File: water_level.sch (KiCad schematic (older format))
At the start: 14 parts, among them U1 LTV-847

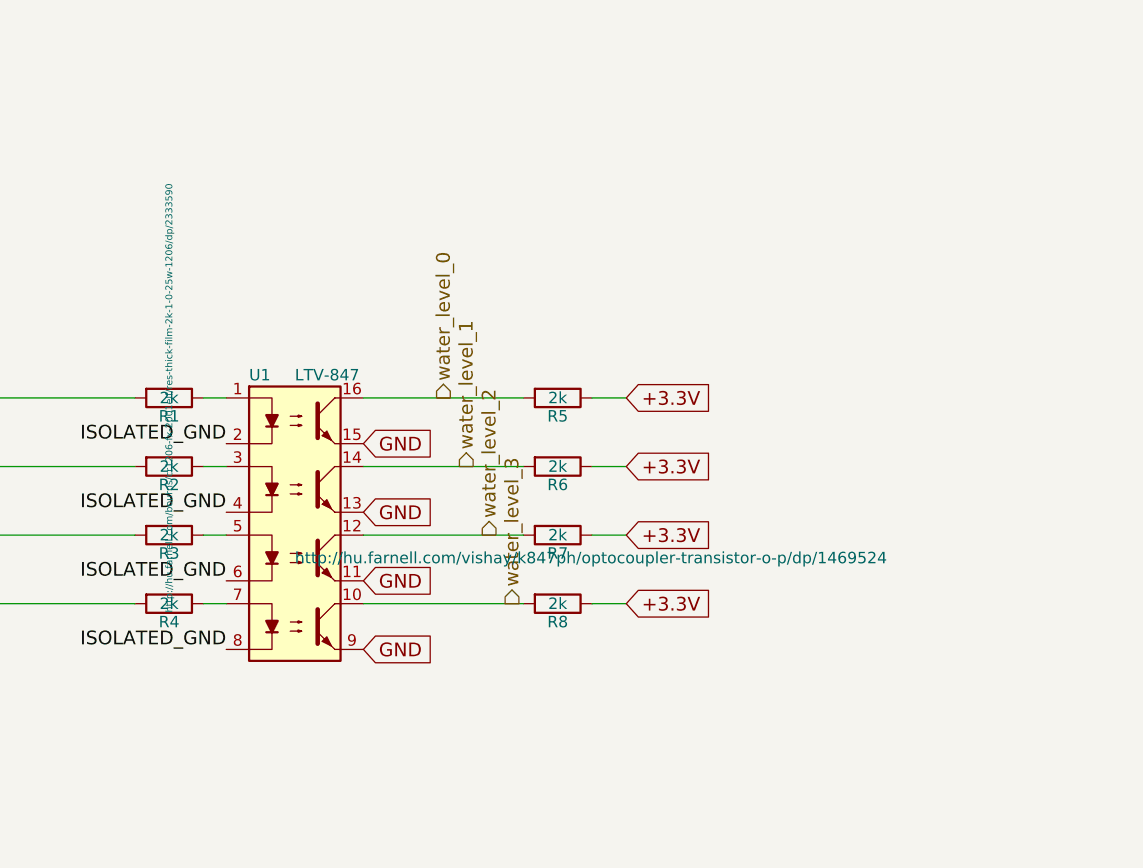
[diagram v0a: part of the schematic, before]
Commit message: stash commit before the revision of the parts
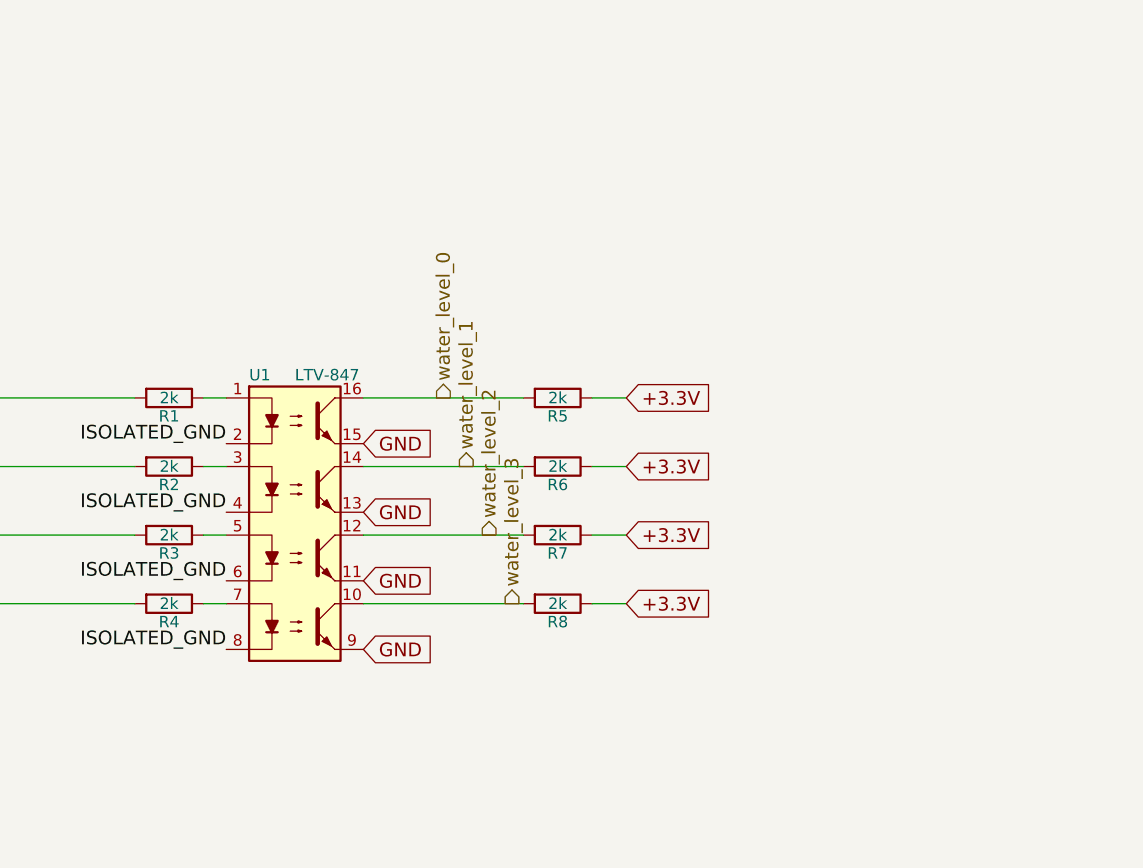
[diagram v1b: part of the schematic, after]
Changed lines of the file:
@@
 F 1 "LTV-847" H 7350 3850 50  0000 L CNN
 F 2 "Housings_SOIC:SOIC-16_3.9x9.9mm_Pitch1.27mm" H 7150 2550 50  0001 L CIN
-F 3 "http://hu.farnell.com/vishay/k847ph/optocoupler-transistor-o-p/dp/1469524" H 7350 3050 50  0000 L CNN
+F 3 "http://hu.farnell.com/vishay/k847ph/optocoupler-transistor-o-p/dp/1469524" H 7350 3050 50  0001 L CNN
 	1    7350 3150
 	1    0    0    -1
@@
 F 1 "2k" V 6800 2550 50  0000 C CNN
 F 2 "Resistors_SMD:R_1206_HandSoldering" V 6730 2550 30  0001 C CNN
-F 3 "http://hu.farnell.com/bourns/cr1206-fx-2001elf/res-thick-film-2k-1-0-25w-1206/dp/2333590" H 6800 2550 30  0000 C CNN
+F 3 "http://hu.farnell.com/bourns/cr1206-fx-2001elf/res-thick-film-2k-1-0-25w-1206/dp/2333590" H 6800 2550 30  0001 C CNN
 	1    6800 2550
 	0    1    1    0
@@
 +5V
 $Comp
+L Water_Level_Sensor_Connector SENS_1
+U 1 1 592601C6
+P 3600 2600
+F 0 "SENS_1" H 3450 1500 60  0000 C CNN
+F 1 "Water_Level_Sensor_Connector" H 3600 2600 60  0000 C CNN
+F 2 "Connectors_Terminal_Blocks:TerminalBlock_WAGO-804_RM5mm_5pol" H 3600 2600 60  0001 C CNN
+F 3 "http://hu.farnell.com/wago/2604-1105/tb-wire-to-brd-5pos-12awg/dp/2749668" H 3600 2600 60  0001 C CNN
+	1    3600 2600
+	1    0    0    -1
+$EndComp
+$Comp
+L Water_Level_Sensor_Connector SENS_3
+U 1 1 59260240
+P 3600 5150
+F 0 "SENS_3" H 3450 4050 60  0000 C CNN
+F 1 "Water_Level_Sensor_Connector" H 3600 5150 60  0000 C CNN
+F 2 "Connectors_Terminal_Blocks:TerminalBlock_WAGO-804_RM5mm_5pol" H 3600 5150 60  0001 C CNN
+F 3 "http://hu.farnell.com/wago/2604-1105/tb-wire-to-brd-5pos-12awg/dp/2749668" H 3600 5150 60  0001 C CNN
+	1    3600 5150
+	1    0    0    -1
+$EndComp
+$Comp
+L Water_Level_Sensor_Connector SENS_4
+U 1 1 592602C7
+P 3600 6400
+F 0 "SENS_4" H 3450 5300 60  0000 C CNN
+F 1 "Water_Level_Sensor_Connector" H 3600 6400 60  0000 C CNN
+F 2 "Connectors_Terminal_Blocks:TerminalBlock_WAGO-804_RM5mm_5pol" H 3600 6400 60  0001 C CNN
+F 3 "http://hu.farnell.com/wago/2604-1105/tb-wire-to-brd-5pos-12awg/dp/2749668" H 3600 6400 60  0001 C CNN
+	1    3600 6400
+	1    0    0    -1
+$EndComp
+Wire Wire Line
+	7650 2550 8350 2550
+Wire Wire Line
+	7650 2850 8350 2850
+Wire Wire Line
+	7650 3150 8350 3150
+Wire Wire Line
+	7650 3450 8350 3450
+Wire Wire Line
+	8800 2550 8650 2550
+Wire Wire Line
+	8800 2850 8650 2850
+Wire Wire Line
+	8800 3150 8650 3150
+Wire Wire Line
+	8800 3450 8650 3450
+Wire Wire Line
+	6950 3450 7050 3450
+Wire Wire Line
+	6950 3150 7050 3150
+Wire Wire Line
+	6950 2850 7050 2850
+Wire Wire Line
+	6950 2550 7050 2550
+Text GLabel 7650 3650 2    60   Input ~ 0
+GND
+Text GLabel 7650 3350 2    60   Input ~ 0
+GND
+Text GLabel 7650 3050 2    60   Input ~ 0
+GND
+Text GLabel 7650 2750 2    60   Input ~ 0
+GND
+Text GLabel 8800 2550 2    60   Input ~ 0
++3.3V
+Text GLabel 8800 2850 2    60   Input ~ 0
++3.3V
+Text GLabel 8800 3150 2    60   Input ~ 0
++3.3V
+Text GLabel 8800 3450 2    60   Input ~ 0
++3.3V
+Text Label 2000 1200 0    60   ~ 0
+ISOLATED_GND
+Text Label 3100 2850 2    60   ~ 0
+ISOLATED_GND
+Text Label 3100 4100 2    60   ~ 0
+ISOLATED_GND
+Text Label 3100 5400 2    60   ~ 0
+ISOLATED_GND
+Text Label 3100 6650 2    60   ~ 0
+ISOLATED_GND
+Text Label 7050 2750 2    60   ~ 0
+ISOLATED_GND
+Text Label 7050 3050 2    60   ~ 0
+ISOLATED_GND
+Text Label 7050 3350 2    60   ~ 0
+ISOLATED_GND
+Text Label 7050 3650 2    60   ~ 0
+ISOLATED_GND
+Text Label 2000 1450 0    60   ~ 0
+ISOLATED_+12V
+Text Label 3100 3000 2    60   ~ 0
+ISOLATED_+12V
+Text Label 3100 4250 2    60   ~ 0
+ISOLATED_+12V
+Text Label 3100 5550 2    60   ~ 0
+ISOLATED_+12V
+Text Label 3100 6800 2    60   ~ 0
+ISOLATED_+12V
+Text Label 3100 3150 2    60   ~ 0
+ISOLATED_+12V
+Text Label 3100 4400 2    60   ~ 0
+ISOLATED_+12V
+Text Label 3100 5700 2    60   ~ 0
+ISOLATED_+12V
+Text Label 3100 6950 2    60   ~ 0
+ISOLATED_+12V
+Wire Wire Line
+	3800 3300 4650 3300
+Wire Wire Line
+	4650 3300 4650 2550
+Wire Wire Line
+	4650 2550 6650 2550
+Wire Wire Line
+	3800 4550 4850 4550
+Wire Wire Line
+	4850 4550 4850 2850
+Wire Wire Line
+	4850 2850 6650 2850
+Wire Wire Line
+	3800 5850 5050 5850
+Wire Wire Line
+	5050 5850 5050 3150
+Wire Wire Line
+	5050 3150 6650 3150
+Wire Wire Line
+	3800 7100 5250 7100
+Wire Wire Line
+	5250 7100 5250 3450
+Wire Wire Line
+	5250 3450 6650 3450
+$Comp
 L Water_Level_Sensor_Connector SENS_2
 U 1 1 5925F963
@@
 F 1 "Water_Level_Sensor_Connector" H 3600 3850 60  0000 C CNN
 F 2 "Connectors_Terminal_Blocks:TerminalBlock_WAGO-804_RM5mm_5pol" H 3600 3850 60  0001 C CNN
-F 3 "http://hu.farnell.com/wago/2092-1375/terminal-block-wire-to-brd-5pos/dp/2352416" H 3600 3850 60  0001 C CNN
+F 3 "http://hu.farnell.com/wago/2604-1105/tb-wire-to-brd-5pos-12awg/dp/2749668" H 3600 3850 60  0001 C CNN
 	1    3600 3850
 	1    0    0    -1
 $EndComp
-$Comp
-L Water_Level_Sensor_Connector SENS_1
-U 1 1 592601C6
-P 3600 2600
-F 0 "SENS_1" H 3450 1500 60  0000 C CNN
-F 1 "Water_Level_Sensor_Connector" H 3600 2600 60  0000 C CNN
-F 2 "Connectors_Terminal_Blocks:TerminalBlock_WAGO-804_RM5mm_5pol" H 3600 2600 60  0001 C CNN
-F 3 "http://hu.farnell.com/wago/2092-1375/terminal-block-wire-to-brd-5pos/dp/2352416" H 3600 2600 60  0001 C CNN
-	1    3600 2600
-	1    0    0    -1
-$EndComp
-$Comp
-L Water_Level_Sensor_Connector SENS_3
-U 1 1 59260240
-P 3600 5150
-F 0 "SENS_3" H 3450 4050 60  0000 C CNN
-F 1 "Water_Level_Sensor_Connector" H 3600 5150 60  0000 C CNN
-F 2 "Connectors_Terminal_Blocks:TerminalBlock_WAGO-804_RM5mm_5pol" H 3600 5150 60  0001 C CNN
-F 3 "http://hu.farnell.com/wago/2092-1375/terminal-block-wire-to-brd-5pos/dp/2352416" H 3600 5150 60  0001 C CNN
-	1    3600 5150
-	1    0    0    -1
-$EndComp
-$Comp
-L Water_Level_Sensor_Connector SENS_4
-U 1 1 592602C7
-P 3600 6400
-F 0 "SENS_4" H 3450 5300 60  0000 C CNN
-F 1 "Water_Level_Sensor_Connector" H 3600 6400 60  0000 C CNN
-F 2 "Connectors_Terminal_Blocks:TerminalBlock_WAGO-804_RM5mm_5pol" H 3600 6400 60  0001 C CNN
-F 3 "http://hu.farnell.com/wago/2092-1375/terminal-block-wire-to-brd-5pos/dp/2352416" H 3600 6400 60  0001 C CNN
-	1    3600 6400
-	1    0    0    -1
-$EndComp
-Wire Wire Line
-	7650 2550 8350 2550
-Wire Wire Line
-	7650 2850 8350 2850
-Wire Wire Line
-	7650 3150 8350 3150
-Wire Wire Line
-	7650 3450 8350 3450
-Wire Wire Line
-	8800 2550 8650 2550
-Wire Wire Line
-	8800 2850 8650 2850
-Wire Wire Line
-	8800 3150 8650 3150
-Wire Wire Line
-	8800 3450 8650 3450
-Wire Wire Line
-	6950 3450 7050 3450
-Wire Wire Line
-	6950 3150 7050 3150
-Wire Wire Line
-	6950 2850 7050 2850
-Wire Wire Line
-	6950 2550 7050 2550
-Text GLabel 7650 3650 2    60   Input ~ 0
-GND
-Text GLabel 7650 3350 2    60   Input ~ 0
-GND
-Text GLabel 7650 3050 2    60   Input ~ 0
-GND
-Text GLabel 7650 2750 2    60   Input ~ 0
-GND
-Text GLabel 8800 2550 2    60   Input ~ 0
-+3.3V
-Text GLabel 8800 2850 2    60   Input ~ 0
-+3.3V
-Text GLabel 8800 3150 2    60   Input ~ 0
-+3.3V
-Text GLabel 8800 3450 2    60   Input ~ 0
-+3.3V
-Text Label 2000 1200 0    60   ~ 0
-ISOLATED_GND
-Text Label 3100 2850 2    60   ~ 0
-ISOLATED_GND
-Text Label 3100 4100 2    60   ~ 0
-ISOLATED_GND
-Text Label 3100 5400 2    60   ~ 0
-ISOLATED_GND
-Text Label 3100 6650 2    60   ~ 0
-ISOLATED_GND
-Text Label 7050 2750 2    60   ~ 0
-ISOLATED_GND
-Text Label 7050 3050 2    60   ~ 0
-ISOLATED_GND
-Text Label 7050 3350 2    60   ~ 0
-ISOLATED_GND
-Text Label 7050 3650 2    60   ~ 0
-ISOLATED_GND
-Text Label 2000 1450 0    60   ~ 0
-ISOLATED_+12V
-Text Label 3100 3000 2    60   ~ 0
-ISOLATED_+12V
-Text Label 3100 4250 2    60   ~ 0
-ISOLATED_+12V
-Text Label 3100 5550 2    60   ~ 0
-ISOLATED_+12V
-Text Label 3100 6800 2    60   ~ 0
-ISOLATED_+12V
-Text Label 3100 3150 2    60   ~ 0
-ISOLATED_+12V
-Text Label 3100 4400 2    60   ~ 0
-ISOLATED_+12V
-Text Label 3100 5700 2    60   ~ 0
-ISOLATED_+12V
-Text Label 3100 6950 2    60   ~ 0
-ISOLATED_+12V
-Wire Wire Line
-	3800 3300 4650 3300
-Wire Wire Line
-	4650 3300 4650 2550
-Wire Wire Line
-	4650 2550 6650 2550
-Wire Wire Line
-	3800 4550 4850 4550
-Wire Wire Line
-	4850 4550 4850 2850
-Wire Wire Line
-	4850 2850 6650 2850
-Wire Wire Line
-	3800 5850 5050 5850
-Wire Wire Line
-	5050 5850 5050 3150
-Wire Wire Line
-	5050 3150 6650 3150
-Wire Wire Line
-	3800 7100 5250 7100
-Wire Wire Line
-	5250 7100 5250 3450
-Wire Wire Line
-	5250 3450 6650 3450
 $EndSCHEMATC
